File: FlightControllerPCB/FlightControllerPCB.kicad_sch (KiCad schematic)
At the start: 0 parts

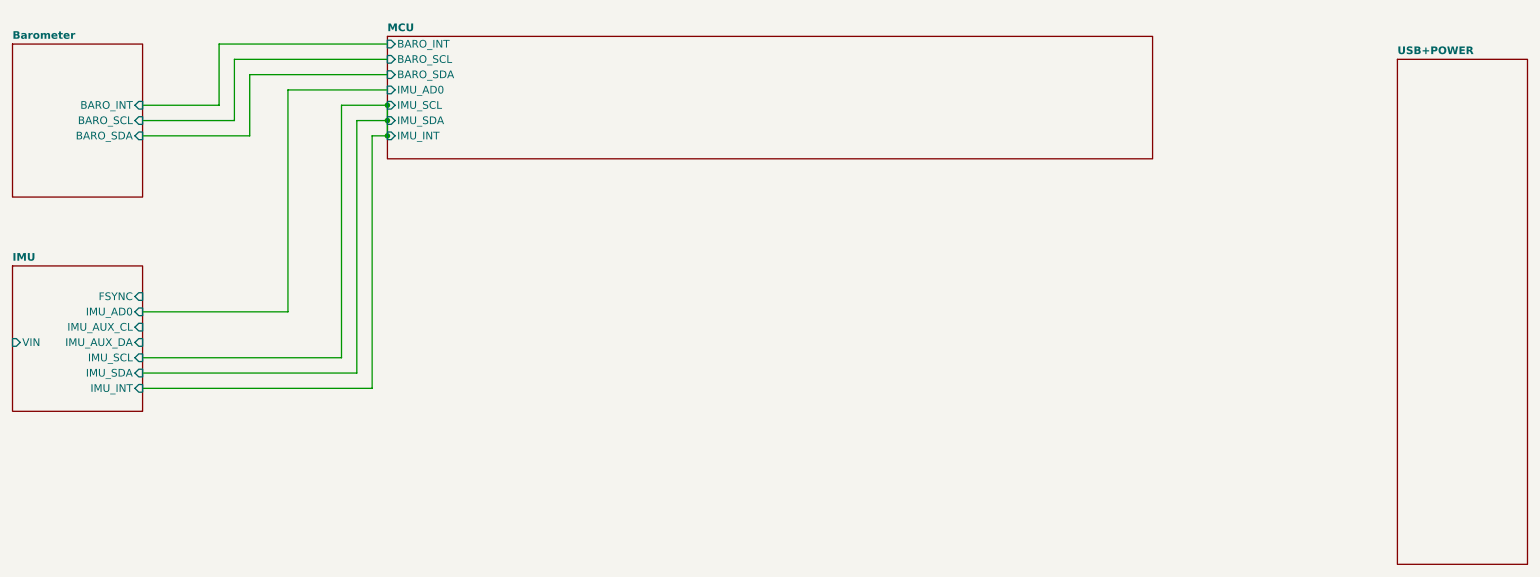
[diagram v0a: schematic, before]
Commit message: actually the IMU+baro changes
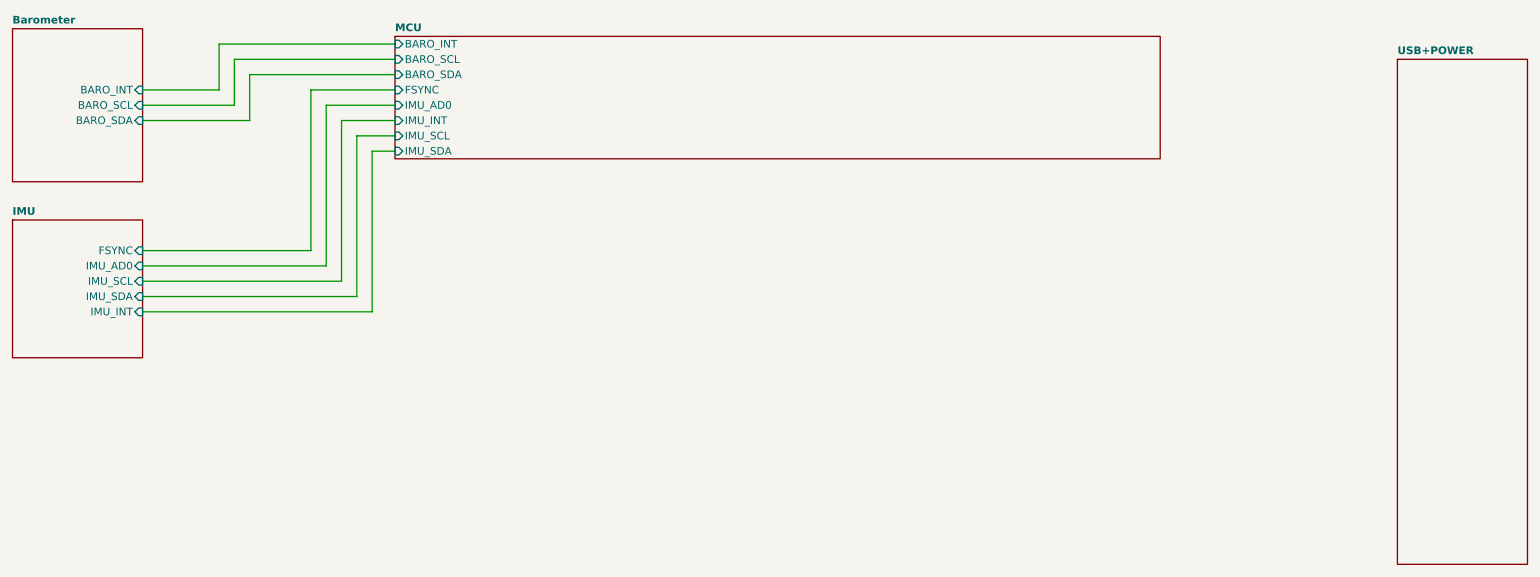
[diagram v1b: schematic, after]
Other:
- sheet IMU ports: added none; removed IMU_AUX_CL, IMU_AUX_DA, VIN
- sheet MCU ports: added FSYNC; removed none
